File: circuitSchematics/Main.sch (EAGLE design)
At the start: 9 parts, among them J1 RASPBERRYPI-40-PIN-GPIO_PTH, J2 Heating_element, Q1 60V/32A/35mΩ, U1 DS18B20

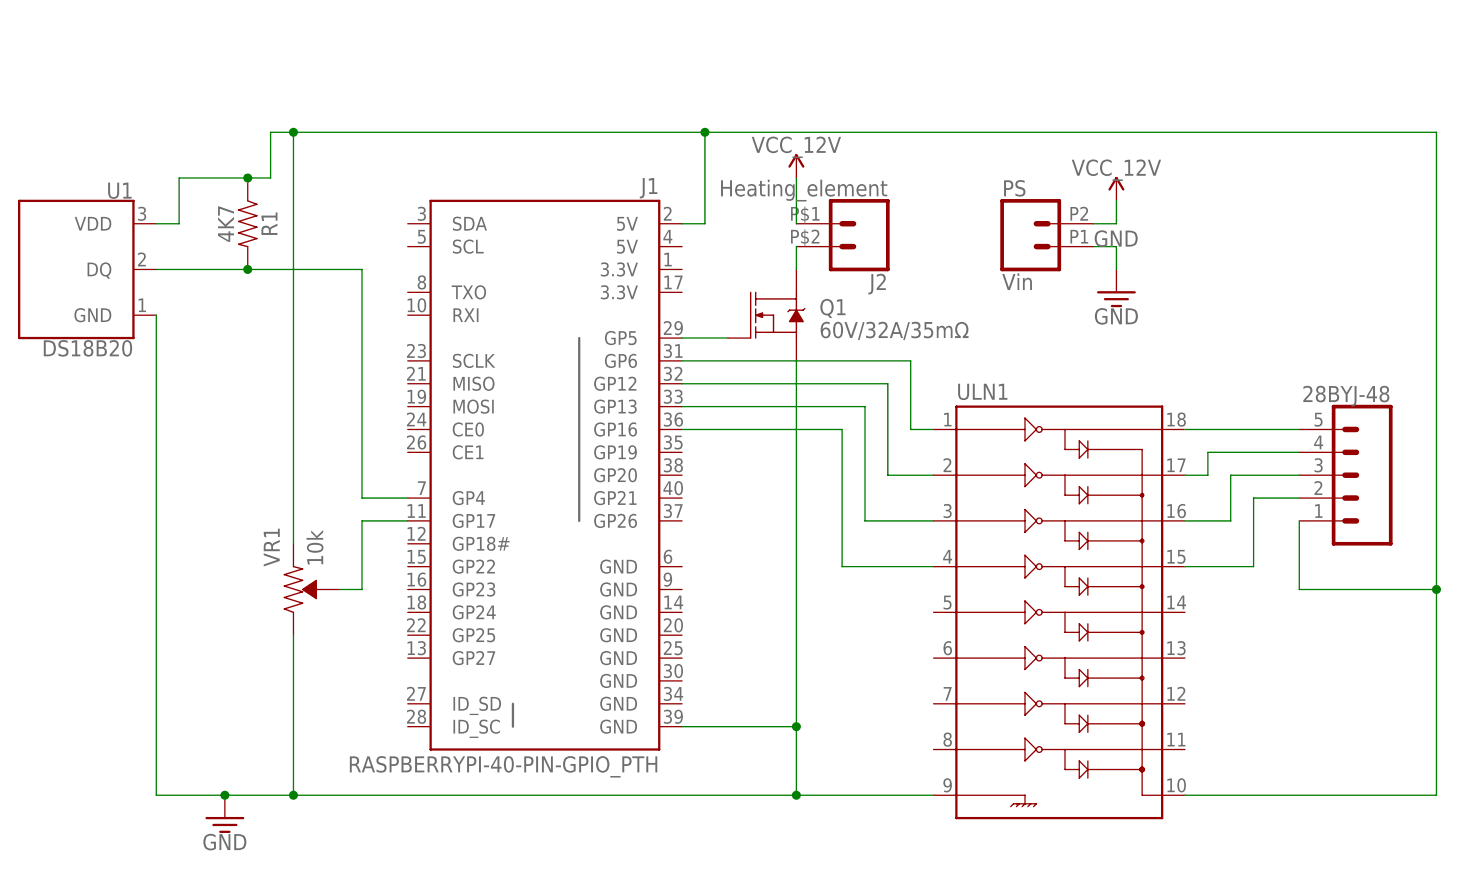
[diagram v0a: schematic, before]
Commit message: Updated circuit schematics
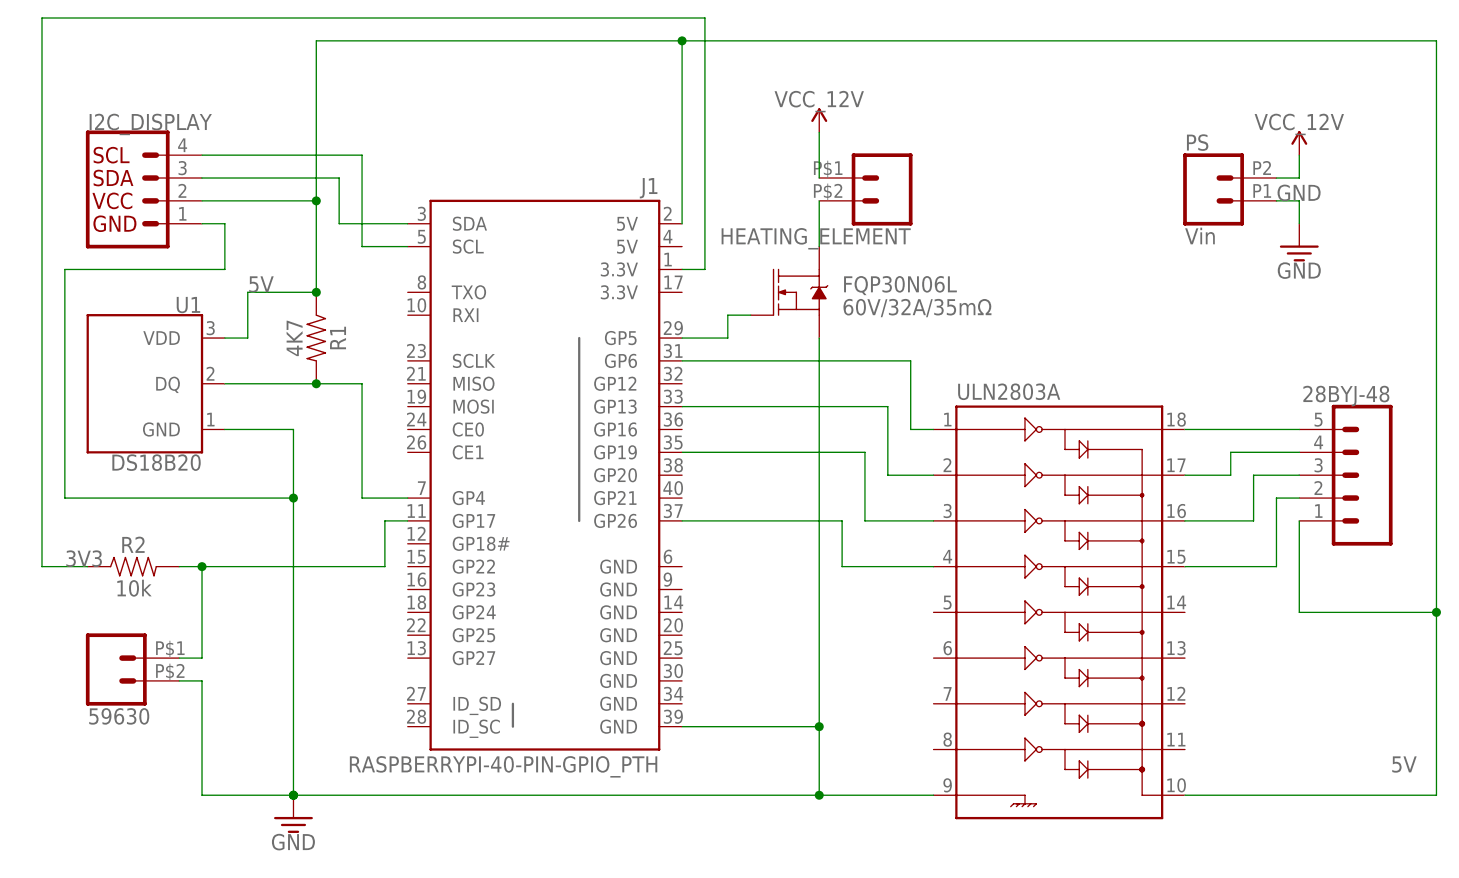
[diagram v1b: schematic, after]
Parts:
- removed J2: Heating_element, SparkFun-Connectors:CONN_02PTH2
- removed Q1: 60V/32A/35mΩ, SparkFun-DiscreteSemi:MOSFET-NCH-FQP30N06L
- removed VR1: 10k, SparkFun-Resistors:TRIMPOT-PTH-10MM-KNOB-1/2W-10%
- added 59630, HEATING_ELEMENT: (no value), SparkFun-Connectors:CONN_02PTH2
- added FQP30N06L: 60V/32A/35mΩ, SparkFun-DiscreteSemi:MOSFET-NCH-FQP30N06L
- added I2C_DISPLAY: (no value), SparkFun-Connectors:I2C_STANDARD
- added R2: 10k, SparkFun-Resistors:10KOHM-HORIZ-1/4W-1%
- renumbered ULN1 to ULN2803A
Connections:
- net N$1 renamed DQ
- removed net N$12: J1.GP16, ULN2803A.4
- removed net N$7: J1.GP17, VR1.WIPER
- removed net VCC_12V: J2.1, PS.2
- new net 12V: HEATING_ELEMENT.1, PS.2
- new net 3V3: J1.3.3V@1, R2.1
- new net N$5: J1.GP26, ULN2803A.4
- new net SCL: I2C_DISPLAY.4, J1.SCL
- new net SDA: I2C_DISPLAY.3, J1.SDA
- new net WS: 59630.1, J1.GP17, R2.2
- net 5V: now also I2C_DISPLAY.2; no longer VR1.CCW
- net GND: now also 59630.2, FQP30N06L.S, I2C_DISPLAY.1; no longer Q1.S, VR1.CW
- net N$10: now also J1.GP13; no longer J1.GP12
- net N$3: now also FQP30N06L.G; no longer Q1.G
- net N$4: now also J1.GP19; no longer J1.GP13
- net N$8: now also FQP30N06L.D, HEATING_ELEMENT.2; no longer J2.2, Q1.D
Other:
- moved on the sheet: PS, R1, U1
